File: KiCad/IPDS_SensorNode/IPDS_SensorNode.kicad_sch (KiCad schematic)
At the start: 10 parts, among them J1 ESP32_LEFT, J2 ESP32_RIGHT, J3 MPU6050, J4 DS3231_RTC, J5 NEO-6M_GPS, J6 USB_Micro_B

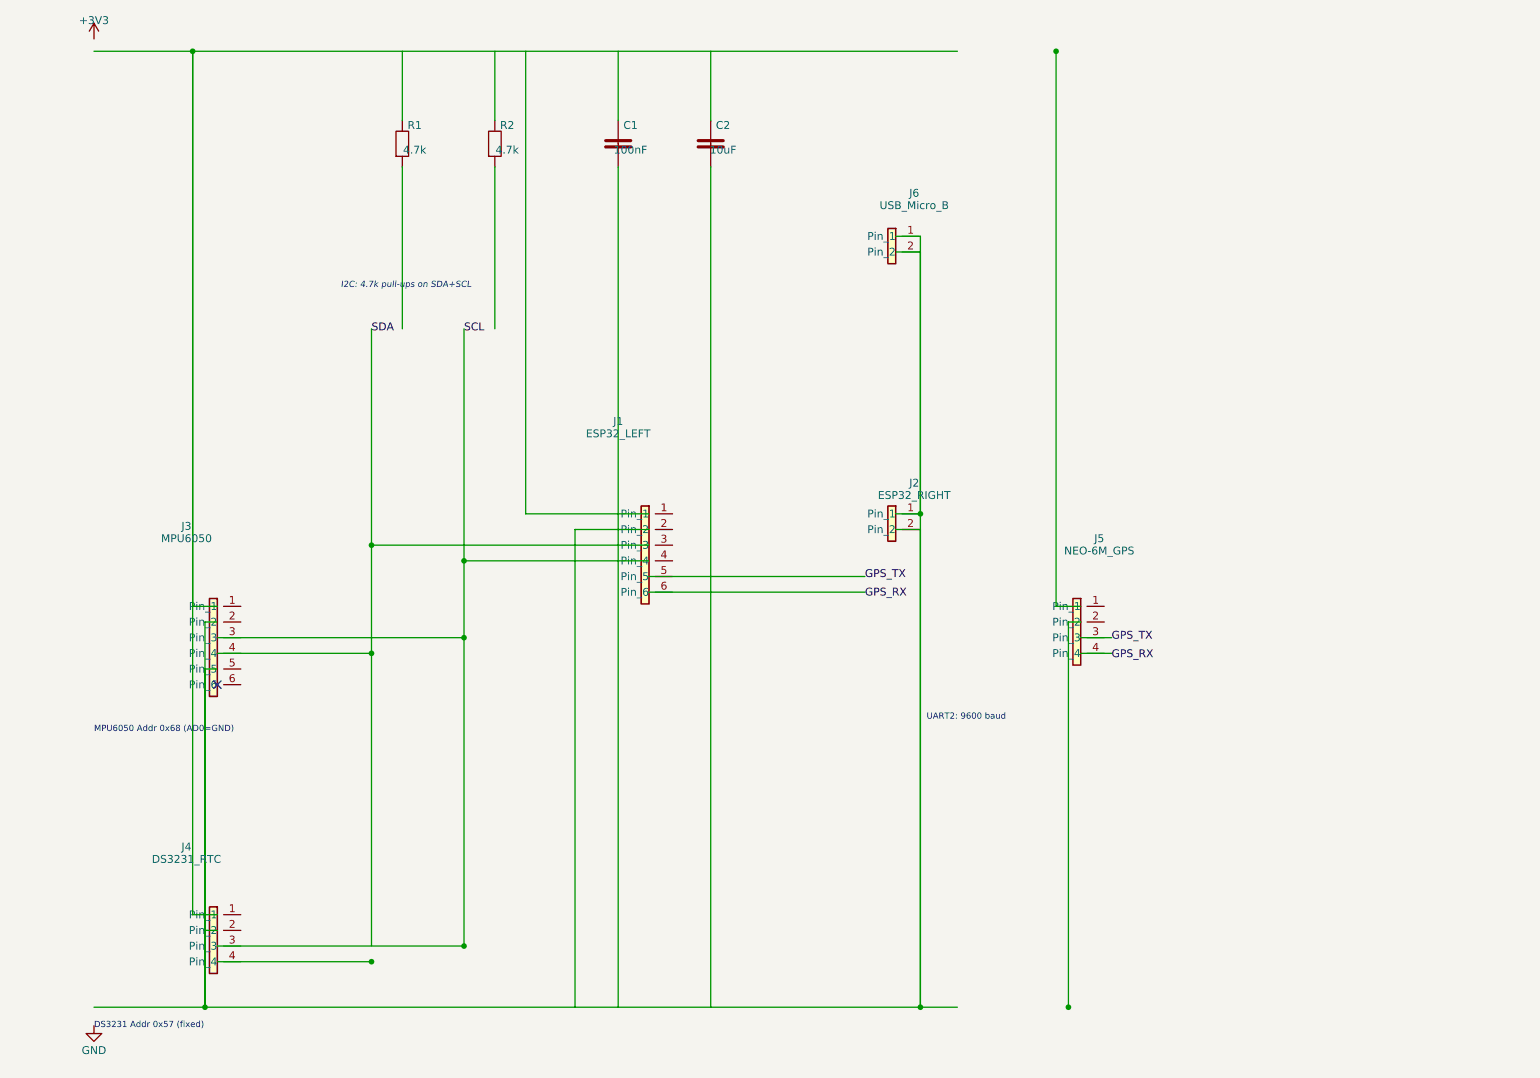
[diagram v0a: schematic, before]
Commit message: Update KiCad sensor node PCB layout, symbol libraries, and fabrication outputs
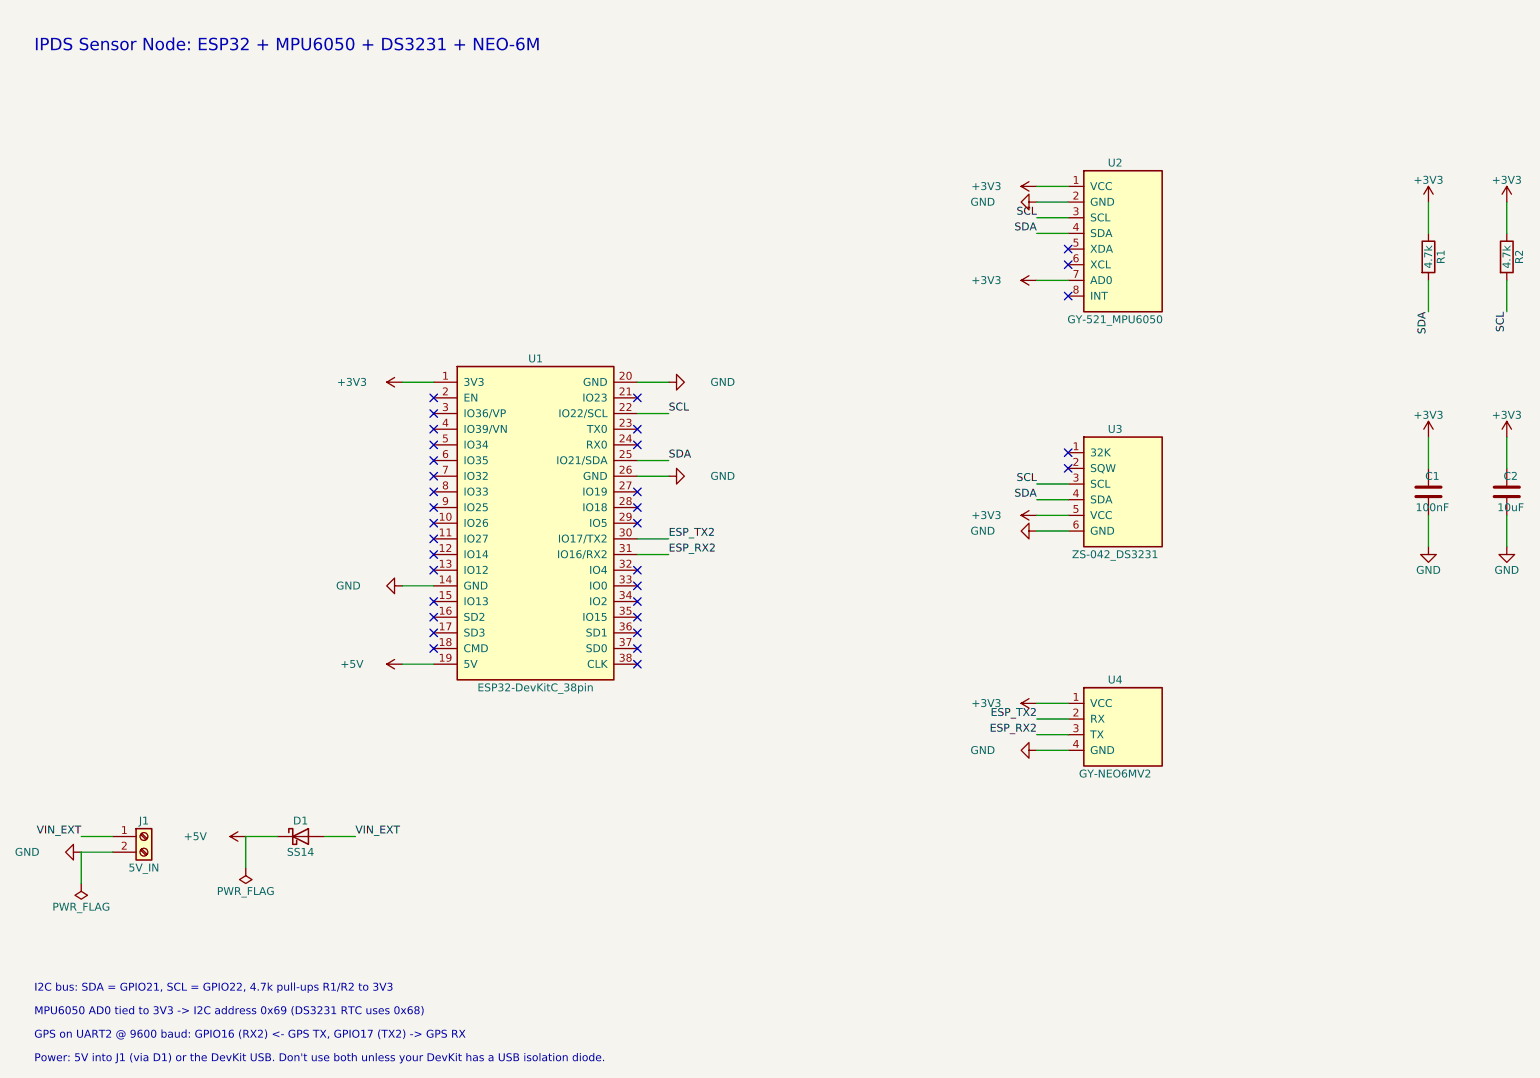
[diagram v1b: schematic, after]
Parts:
- removed J1: ESP32_LEFT, Connector_PinHeader_2.54mm:PinHeader_1x19_P2.54mm_Vertical, symbol Connector_Generic:Conn_01x06
- removed J2: ESP32_RIGHT, Connector_PinHeader_2.54mm:PinHeader_1x19_P2.54mm_Vertical, symbol Connector_Generic:Conn_01x02
- removed J3: MPU6050, Connector_PinHeader_2.54mm:PinHeader_1x06_P2.54mm_Vertical, symbol Connector_Generic:Conn_01x06
- removed J4: DS3231_RTC, Connector_PinHeader_2.54mm:PinHeader_1x04_P2.54mm_Vertical, symbol Connector_Generic:Conn_01x04
- removed J5: NEO-6M_GPS, Connector_PinHeader_2.54mm:PinHeader_1x04_P2.54mm_Vertical, symbol Connector_Generic:Conn_01x04
- removed J6: USB_Micro_B, Connector_USB:USB_Micro-B_Molex_47589-0001, symbol Connector_Generic:Conn_01x02
- added D1: SS14, Diode_SMD:D_SMA, symbol Device:D_Schottky
- added J1: 5V_IN, TerminalBlock_Phoenix:TerminalBlock_Phoenix_MKDS-1,5-2-5.08_1x02_P5.08mm_Horizontal, symbol Connector:Screw_Terminal_01x02
- added U1: ESP32-DevKitC_38pin, IPDS:ESP32_DevKitC_38_Socket, symbol IPDS:ESP32_DevKitC_38
- added U2: GY-521_MPU6050, Connector_PinSocket_2.54mm:PinSocket_1x08_P2.54mm_Vertical, symbol IPDS:GY-521_MPU6050
- added U3: ZS-042_DS3231, Connector_PinSocket_2.54mm:PinSocket_1x06_P2.54mm_Vertical, symbol IPDS:ZS-042_DS3231
- added U4: GY-NEO6MV2, Connector_PinSocket_2.54mm:PinSocket_1x04_P2.54mm_Vertical, symbol IPDS:GY-NEO6MV2
- C1: footprint Capacitor_SMD:C_0402_1005Metric -> Capacitor_SMD:C_0805_2012Metric
- R1, R2: footprint Resistor_SMD:R_0402_1005Metric -> Resistor_SMD:R_0805_2012Metric
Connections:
- net SCL: now also R2.2, U1.22 (IO22/SCL), U2.3 (SCL), U3.3 (SCL)
- net SDA: now also R1.2, U1.25 (IO21/SDA), U2.4 (SDA), U3.4 (SDA)
- net +3V3: now reaches R1.1
- net +3V3: now also C1.1, C2.1, R2.1, U1.1 (3V3), U2.1 (VCC), U2.7 (AD0), U3.5 (VCC), U4.1 (VCC)
- net GND: now reaches C1.2
- net GND: now also C2.2, J1.2 (Pin_2), U1.14 (GND), U1.20 (GND), U1.26 (GND), U2.2 (GND), U3.6 (GND), U4.4 (GND)
- new net +5V: D1.1 (K), U1.19 (5V)
- new net ESP_RX2: U1.31 (IO16/RX2), U4.3 (TX)
- new net ESP_TX2: U1.30 (IO17/TX2), U4.2 (RX)
- new net VIN_EXT: D1.2 (A), J1.1 (Pin_1)
- no-connect marks 1 -> 34
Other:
- note added: "GPS on UART2 @ 9600 baud: GPIO16 (RX2) <- GPS TX, GPIO17 (TX2) -> GPS RX"
- note added: "I2C bus: SDA = GPIO21, SCL = GPIO22, 4.7k pull-ups R1/R2 to 3V3"
- note added: "IPDS Sensor Node: ESP32 + MPU6050 + DS3231 + NEO-6M"
- note added: "MPU6050 AD0 tied to 3V3 -> I2C address 0x69 (DS3231 RTC uses 0x68)"
- note added: "Power: 5V into J1 (via D1) or the DevKit USB. Don't use both unless your DevKit has a USB isolation diode."
- note removed: "DS3231 Addr 0x57 (fixed)"
- note removed: "I2C: 4.7k pull-ups on SDA+SCL"
- note removed: "MPU6050 Addr 0x68 (AD0=GND)"
- note removed: "UART2: 9600 baud"
